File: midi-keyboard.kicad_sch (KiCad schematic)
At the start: 69 parts, among them J1 Conn_01x04, SW1 SW_Push_45deg, SW10 SW_Push_45deg, SW11 SW_Push_45deg, SW12 SW_Push_45deg, SW13 SW_Push_45deg, SW14 SW_Push_45deg, SW15 SW_Push_45deg, SW16 SW_Push_45deg, SW17 SW_Push_45deg, SW18 SW_Push_45deg, SW19 SW_Push_45deg, SW2 SW_Push_45deg, SW20 SW_Push_45deg, SW21 SW_Push_45deg, SW22 SW_Push_45deg, SW23 SW_Push_45deg, SW24 SW_Push_45deg, SW25 SW_Push_45deg, SW26 SW_Push_45deg, SW27 SW_Push_45deg, SW28 SW_Push_45deg, SW29 SW_Push_45deg, SW3 SW_Push_45deg, SW30 SW_Push_45deg, SW31 SW_Push_45deg, SW32 SW_Push_45deg, SW33 SW_Push_45deg, SW4 SW_Push_45deg, SW44 SW_Push_45deg, SW5 SW_Push_45deg, SW6 SW_Push_45deg, SW7 SW_Push_45deg, SW8 SW_Push_45deg, SW9 SW_Push_45deg

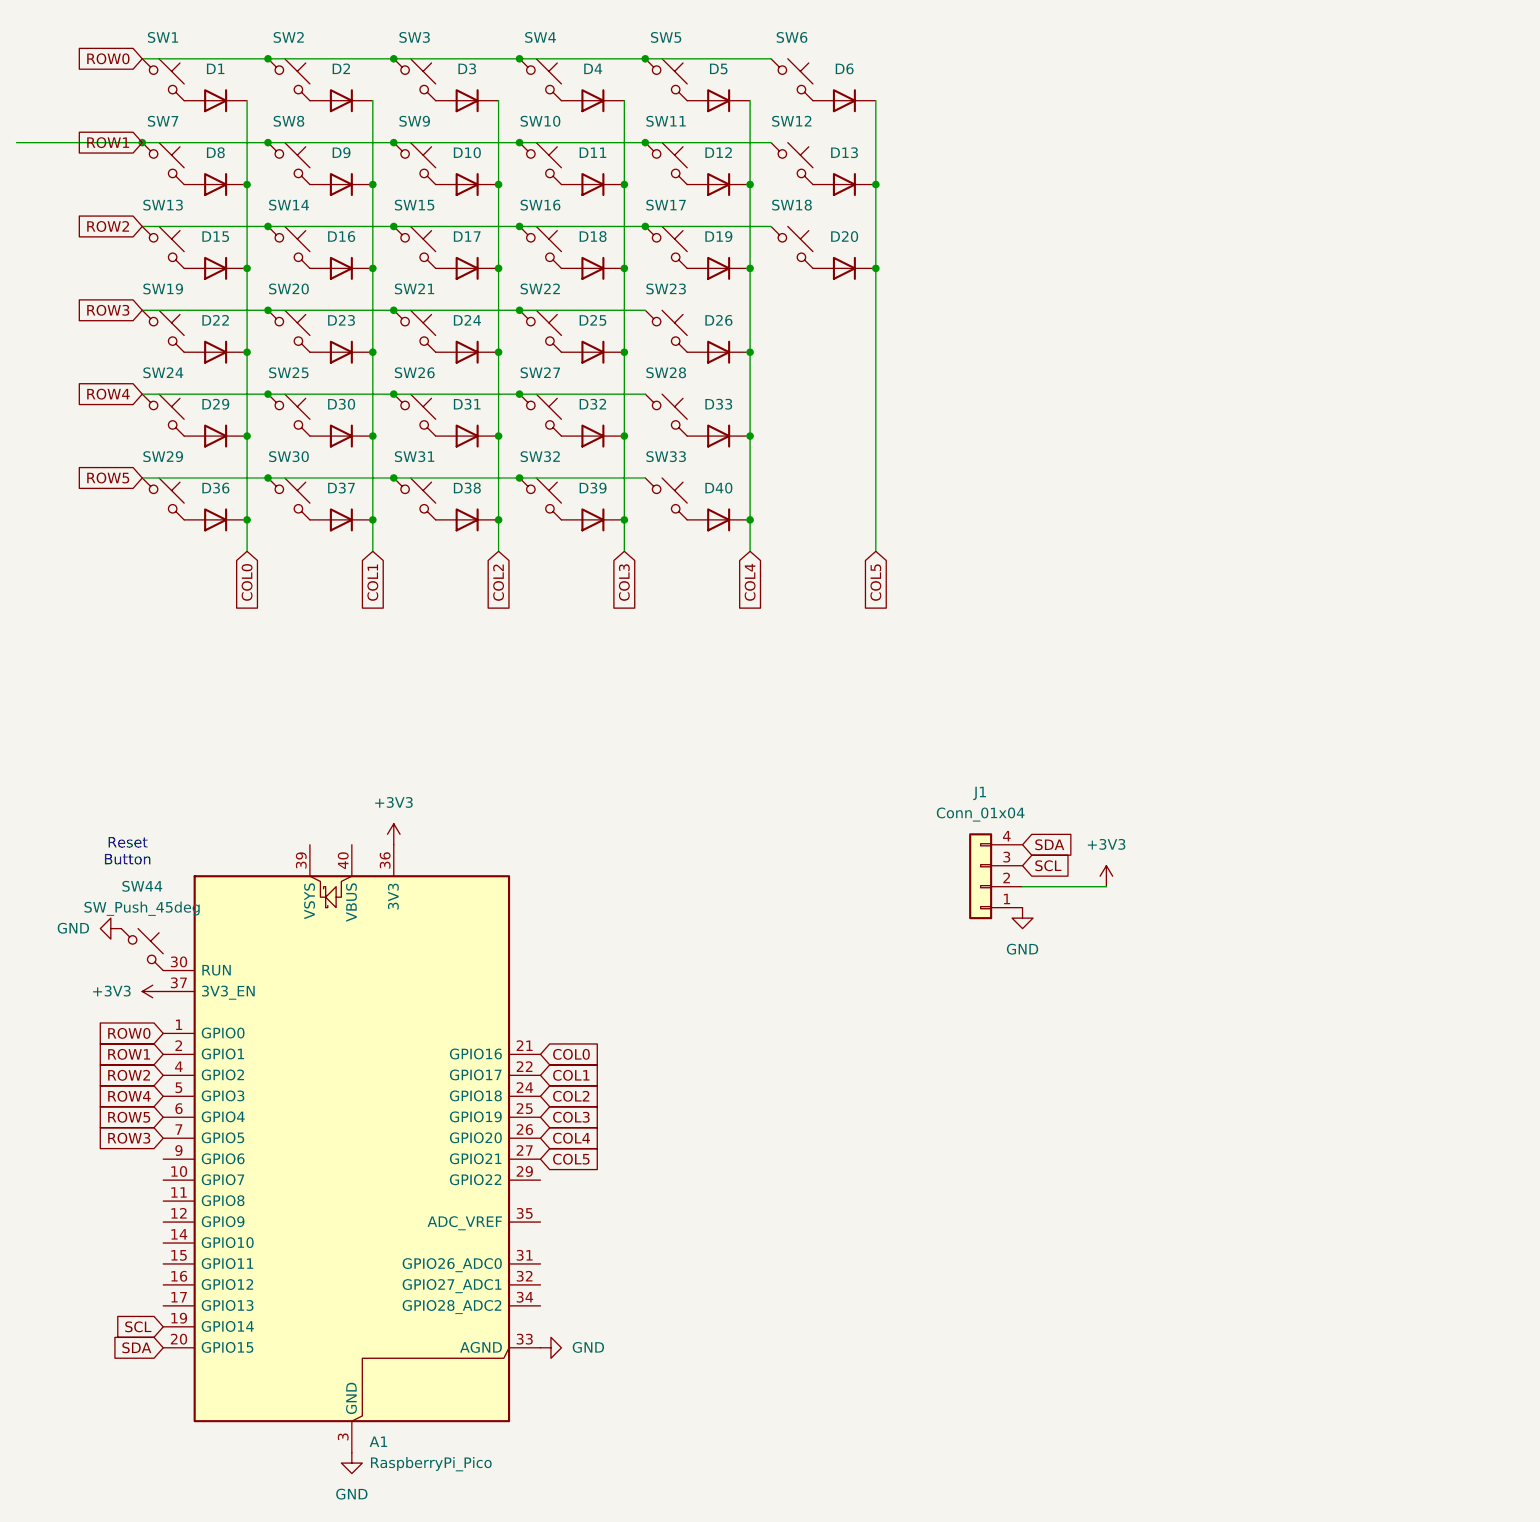
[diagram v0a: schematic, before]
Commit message: README
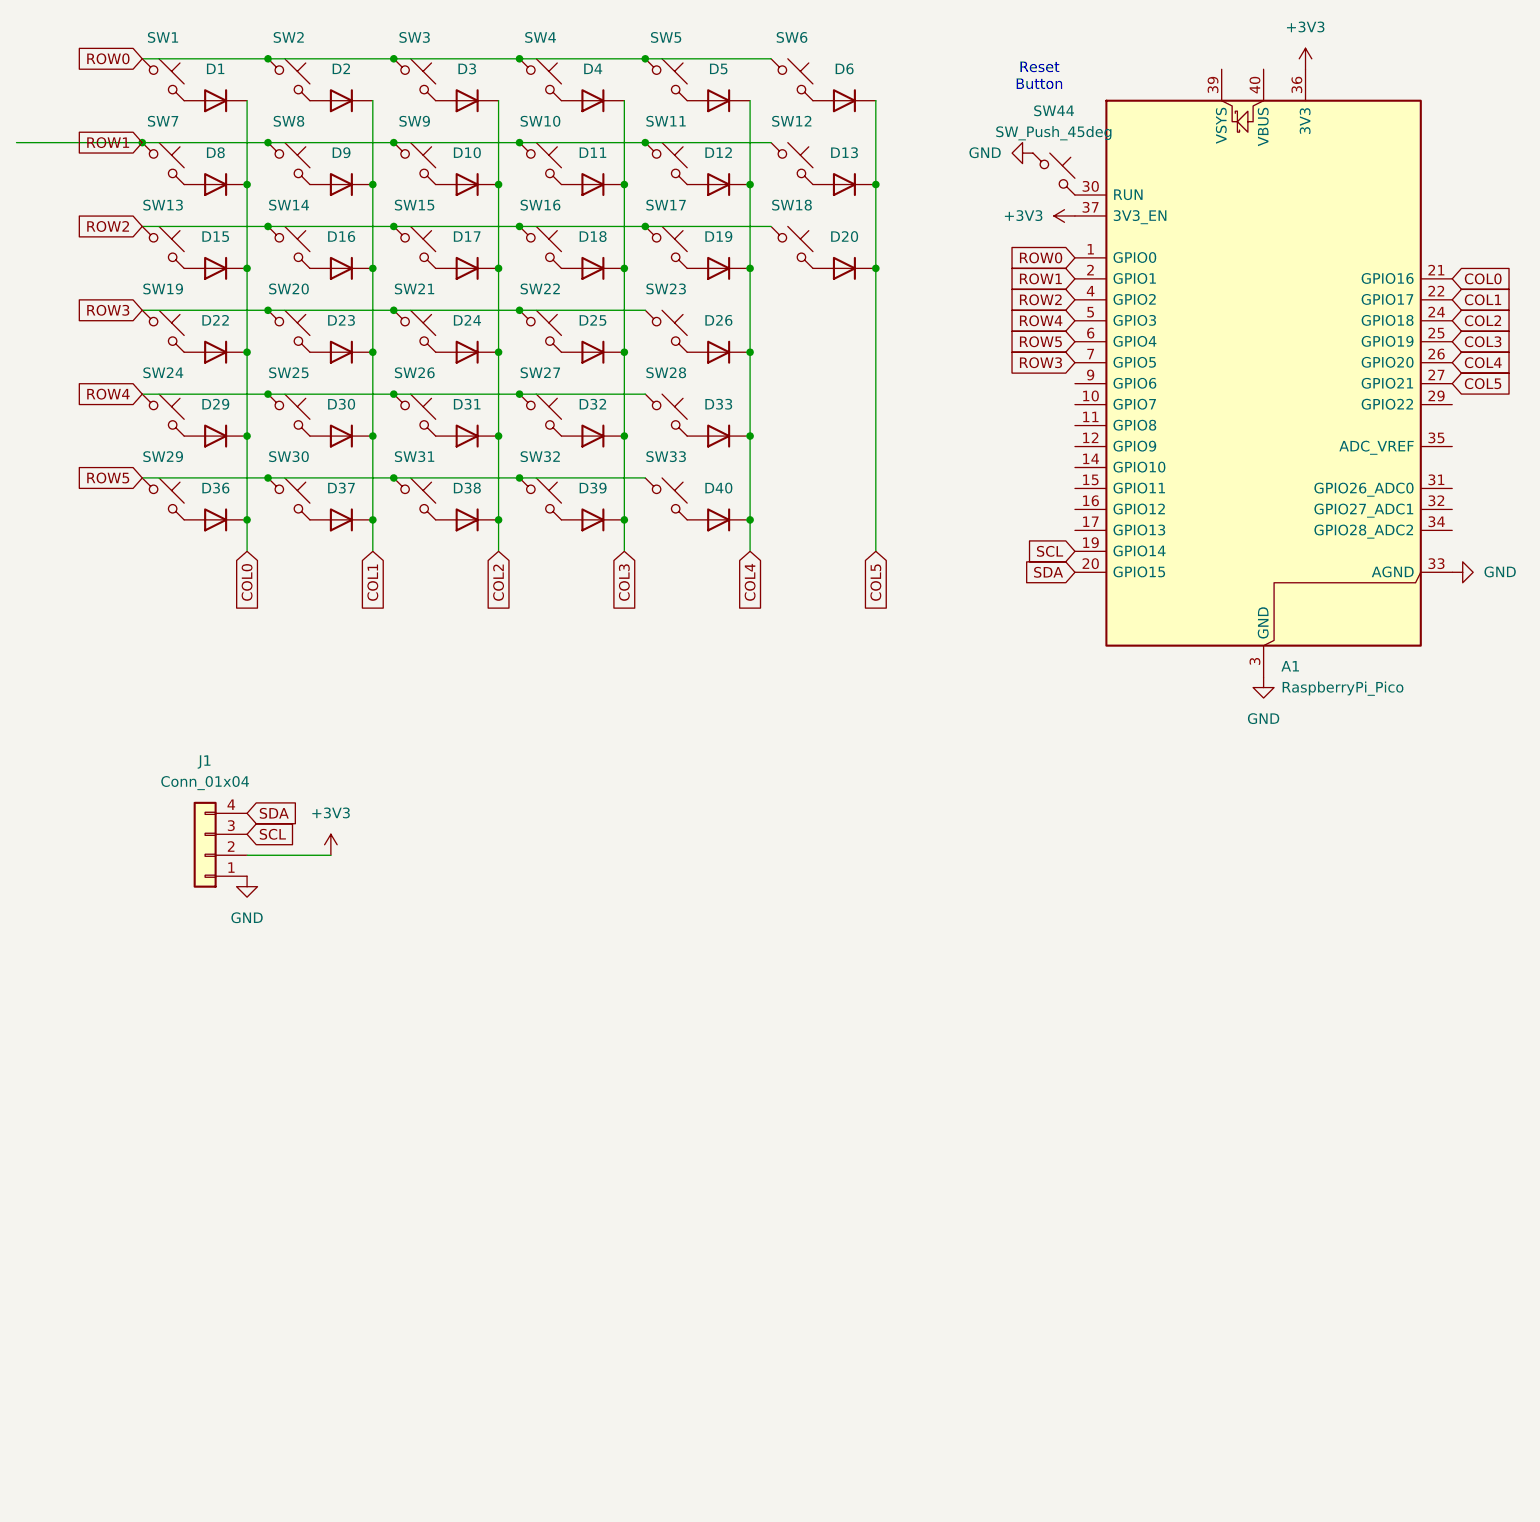
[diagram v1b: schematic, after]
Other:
- title: (none) -> MusePad
- moved on the sheet: A1, J1, SW44
